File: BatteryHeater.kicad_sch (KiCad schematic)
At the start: 15 parts, among them Q5 Si1442DH, Q7 Si1442DH, Q9 Si1442DH

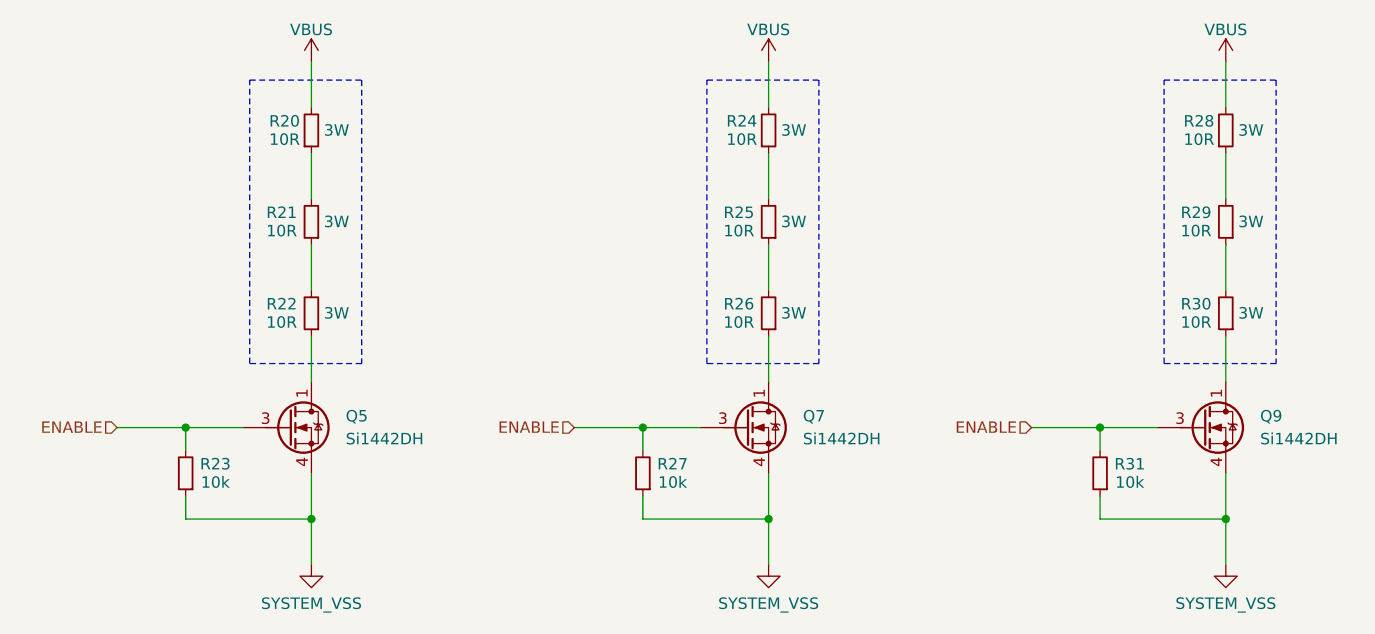
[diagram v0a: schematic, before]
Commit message: More updates
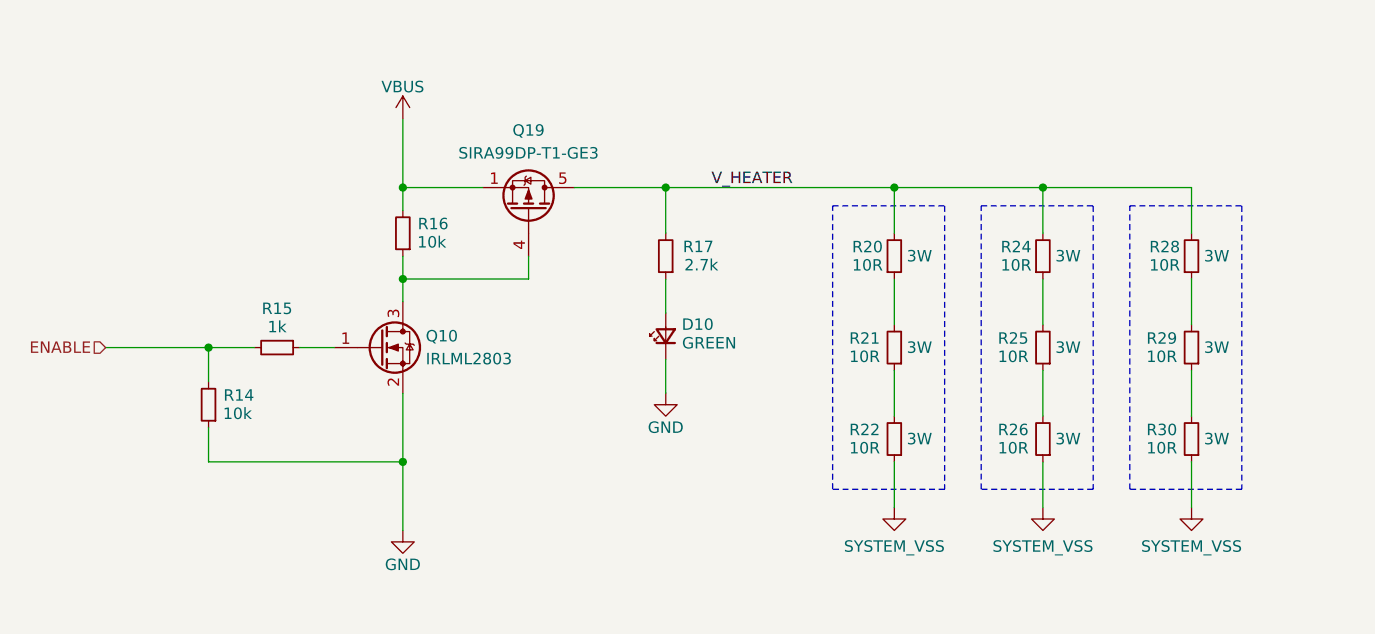
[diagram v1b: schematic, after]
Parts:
- removed Q5, Q7, Q9: Si1442DH, Package_TO_SOT_SMD:SOT-363_SC-70-6, symbol Transistor_FET:Si1442DH
- removed R23, R27, R31: 10k, Resistor_SMD:R_0603_1608Metric, symbol Device:R_Small
- added D10: GREEN, LED_SMD:LED_0603_1608Metric, symbol Device:LED_Small
- added Q10: IRLML2803, Package_TO_SOT_SMD:SOT-23, symbol Argus-IC:IRLML2803
- added Q19: SIRA99DP-T1-GE3, Package_SO:PowerPAK_SO-8_Single, symbol Transistor_FET:Si7141DP
- added R14, R16: 10k, Resistor_SMD:R_0603_1608Metric, symbol Device:R_Small
- added R15: 1k, Resistor_SMD:R_0603_1608Metric, symbol Device:R_Small
- added R17: 2.7k, Resistor_SMD:R_0603_1608Metric, symbol Device:R_Small
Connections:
- net ENABLE: now also R14.2, R15.2
- net SYSTEM_VSS: now also R22.1, R26.1, R30.1
- net VBUS: now also Q19.1 (S), Q19.2 (S), Q19.3 (S), R16.2; no longer R20.2, R24.2, R28.2
- new net: D10.2 (A), R17.1
- new net: Q10.1 (G), R15.1
- new net: Q10.3 (D), Q19.4 (G), R16.1
- new net GND: D10.1 (K), Q10.2 (S), R14.1
- new net V_HEATER: Q19.5 (D), R17.2, R20.2, R24.2, R28.2
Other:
- moved on the sheet: R20, R21, R22, R24, R25, R26, R28, R29, R30

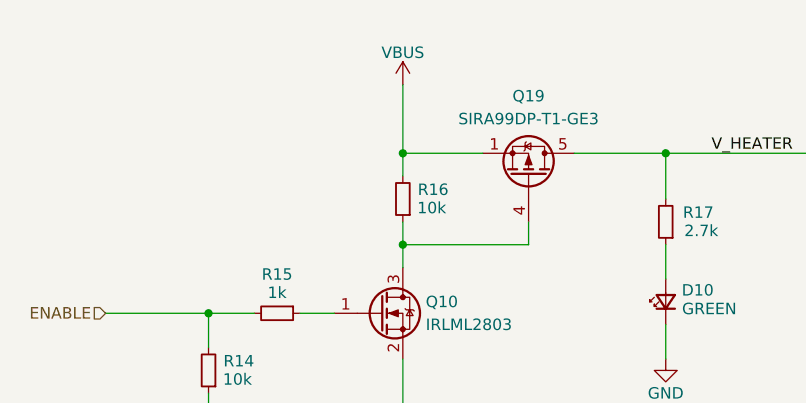
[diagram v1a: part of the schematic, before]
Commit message: Finalized updates with recommendations and exported files
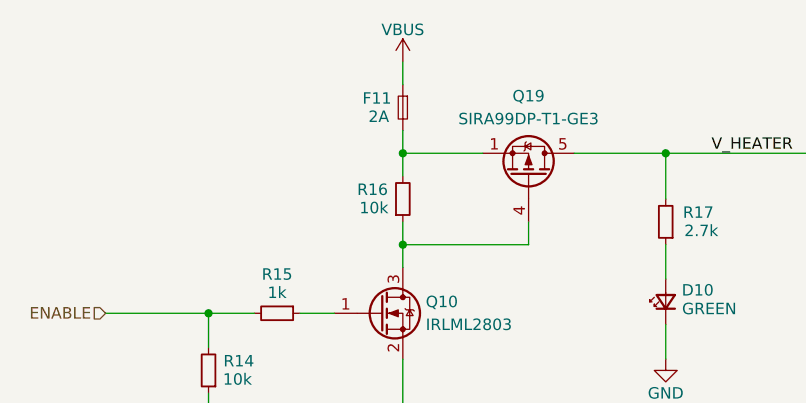
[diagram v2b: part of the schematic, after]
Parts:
- added F11: 2A, Fuse:Fuse_1206_3216Metric, symbol Device:Fuse_Small
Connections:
- net VBUS: now also F11.1; no longer Q19.1 (S), Q19.2 (S), Q19.3 (S), R16.2
- new net: F11.2, Q19.1 (S), Q19.2 (S), Q19.3 (S), R16.2
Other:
- moved on the sheet: R16
